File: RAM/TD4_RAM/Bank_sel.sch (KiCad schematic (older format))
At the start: 2 parts

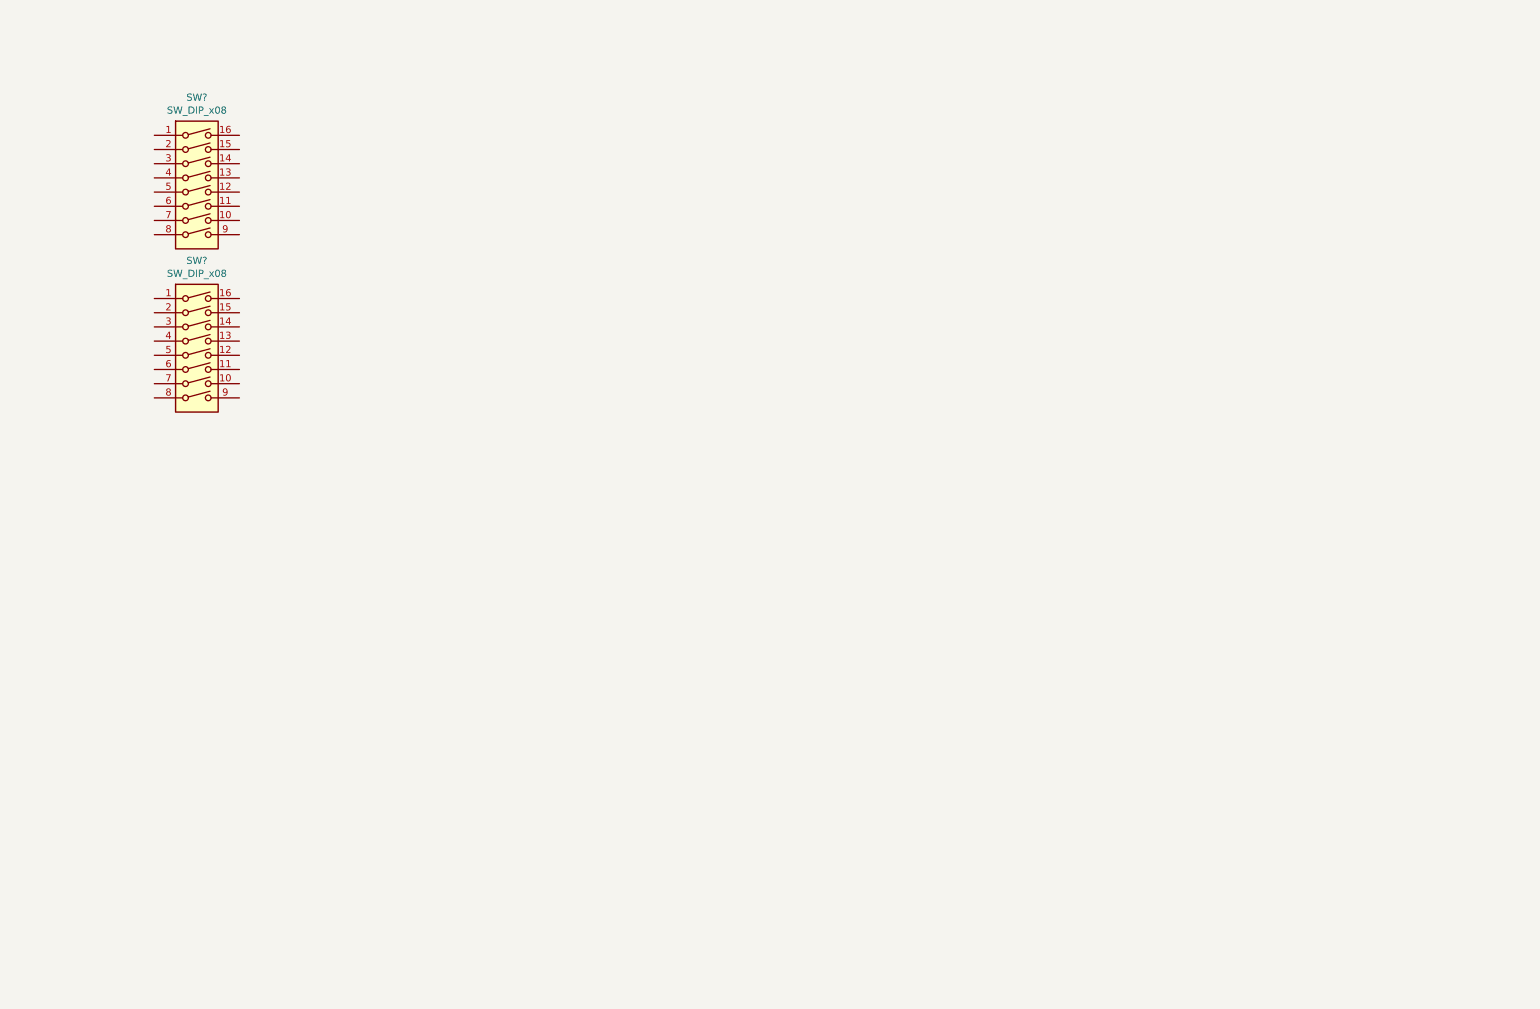
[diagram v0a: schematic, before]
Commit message: RAM done (sort of)
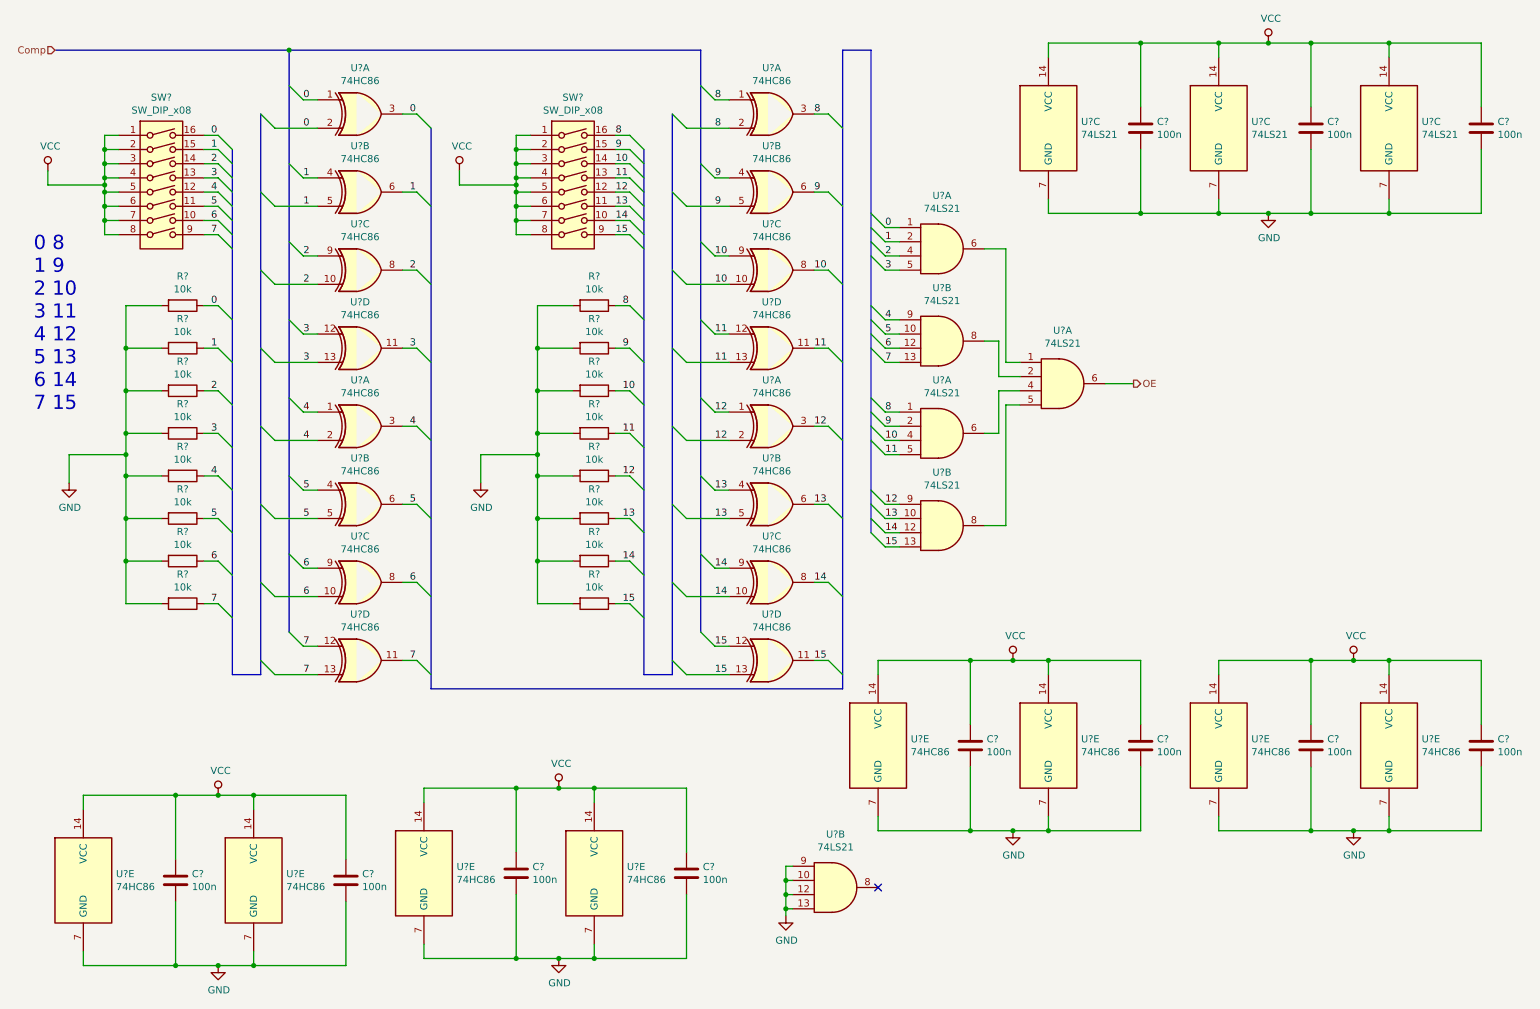
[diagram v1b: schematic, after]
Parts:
- removed SW?: SW_DIP_x08, symbol Switch:SW_DIP_x08
- added C? (x11): 100n, symbol Device:C
- added R? (x16): 10k, symbol Device:R
- added SW?: SW_DIP_x08, symbol Switch:SW_DIP_x08
- added U? (x24): 74HC86, symbol 74xx:74HC86
- added U? (x9): 74LS21, symbol 74xx:74LS21
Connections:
- net VCC: now reaches SW?.1
- net VCC: now also SW?.2, SW?.3, SW?.4, SW?.5, SW?.6, SW?.7, SW?.8, C?.1, C?.1, C?.1, C?.1, C?.1, C?.1, C?.1, C?.1, C?.1, C?.1, C?.1, SW?.1, SW?.2, SW?.3, SW?.4, SW?.5, SW?.6, SW?.7, SW?.8, U?.14 (VCC), U?.14 (VCC), U?.14 (VCC), U?.14 (VCC), U?.14 (VCC), U?.14 (VCC), U?.14 (VCC), U?.14 (VCC), U?.14 (VCC), U?.14 (VCC), U?.14 (VCC)
- net 6: now reaches SW?.10
- net 6: now also R?.1, U?.10, U?.12, U?.8, U?.9
- net 5: now reaches SW?.11
- net 5: now also R?.1, U?.10, U?.4, U?.5, U?.6
- net 4: now reaches SW?.12
- net 4: now also R?.1, U?.1, U?.2, U?.3, U?.9
- net 3: now reaches SW?.13
- net 3: now also R?.1, U?.11, U?.12, U?.13, U?.5
- net 2: now reaches SW?.14
- net 2: now also R?.1, U?.10, U?.4, U?.8, U?.9
- net 1: now reaches SW?.15
- net 1: now also R?.1, U?.2, U?.4, U?.5, U?.6
- net 0: now reaches SW?.16
- net 0: now also R?.1, U?.1, U?.1, U?.2, U?.3
- net 7: now reaches SW?.9
- net 7: now also R?.1, U?.11, U?.12, U?.13, U?.13
- new net: U?.1, U?.6
- new net: U?.2, U?.8
- new net: U?.4, U?.6
- new net: U?.5, U?.8
- new net 10: R?.1, SW?.14, U?.10, U?.4, U?.8, U?.9
- new net 11: R?.1, SW?.13, U?.11, U?.12, U?.13, U?.5
- new net 12: R?.1, SW?.12, U?.1, U?.2, U?.3, U?.9
- new net 13: R?.1, SW?.11, U?.10, U?.4, U?.5, U?.6
- new net 14: R?.1, SW?.10, U?.10, U?.12, U?.8, U?.9
- new net 15: R?.1, SW?.9, U?.11, U?.12, U?.13, U?.13
- new net 8: R?.1, SW?.16, U?.1, U?.1, U?.2, U?.3
- new net 9: R?.1, SW?.15, U?.2, U?.4, U?.5, U?.6
- new net GND: C?.2, C?.2, C?.2, C?.2, C?.2, C?.2, C?.2, C?.2, C?.2, C?.2, C?.2, R?.2, R?.2, R?.2, R?.2, R?.2, R?.2, R?.2, R?.2, R?.2, R?.2, R?.2, R?.2, R?.2, R?.2, R?.2, R?.2, U?.10, U?.12, U?.13, U?.7 (GND), U?.7 (GND), U?.7 (GND), U?.7 (GND), U?.7 (GND), U?.7 (GND), U?.7 (GND), U?.7 (GND), U?.7 (GND), U?.7 (GND), U?.7 (GND), U?.9
- new net OE: U?.6
- no-connect marks 0 -> 1
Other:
- note added: "0 8\n1 9\n2 10\n3 11\n4 12\n5 13\n6 14\n7 15"
- moved on the sheet: SW?
